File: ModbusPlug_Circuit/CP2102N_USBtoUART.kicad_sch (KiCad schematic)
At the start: 10 parts, among them U2 CP2102N-Axx-xQFN20

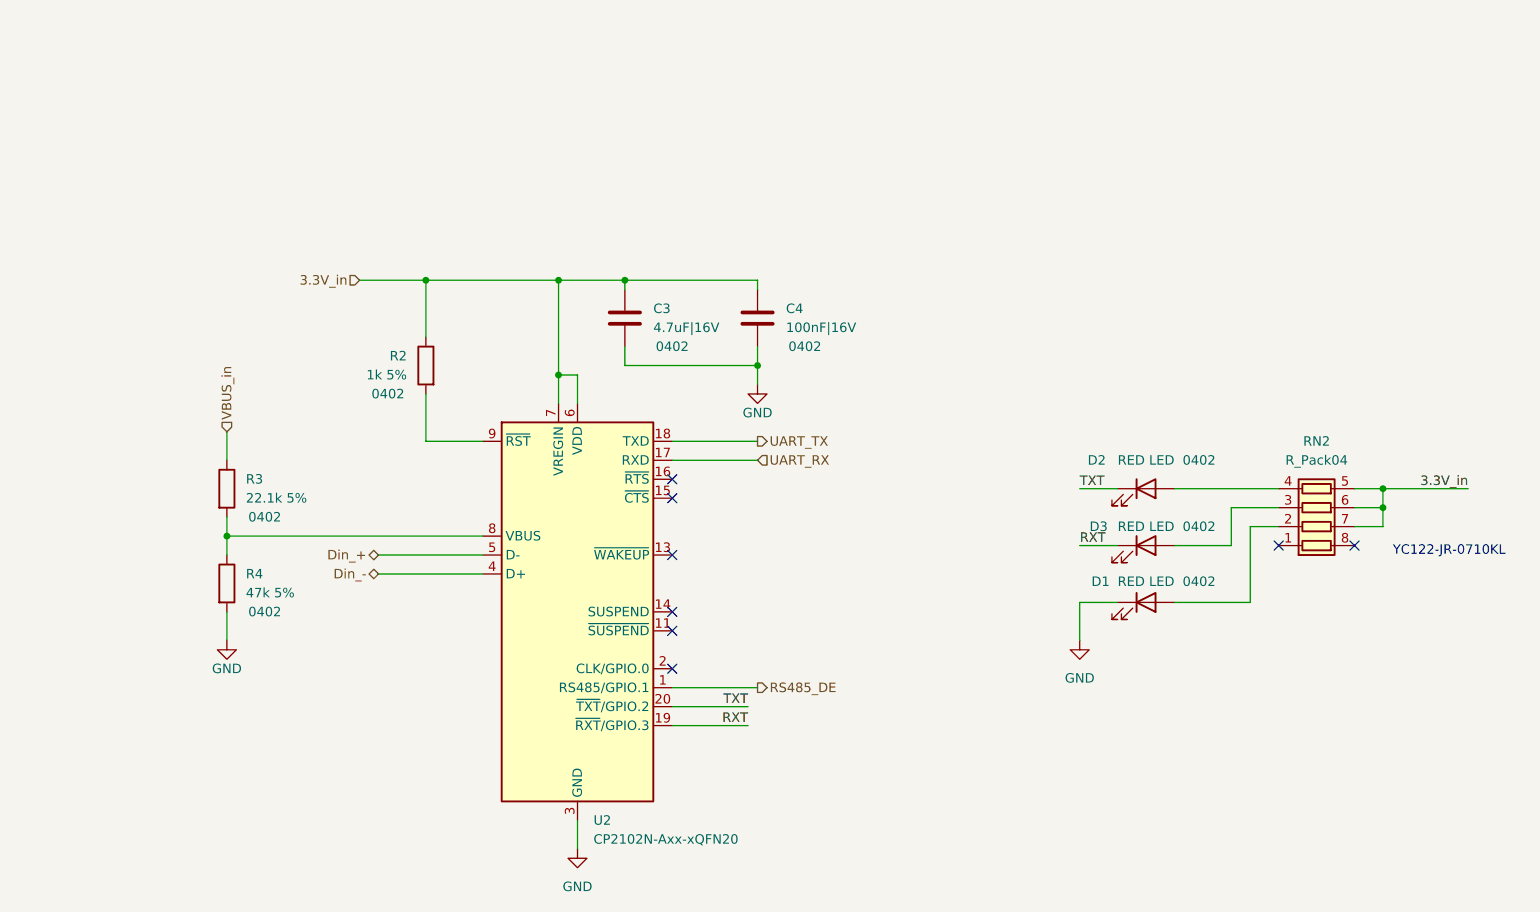
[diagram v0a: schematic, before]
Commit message: pushing V0.1.4
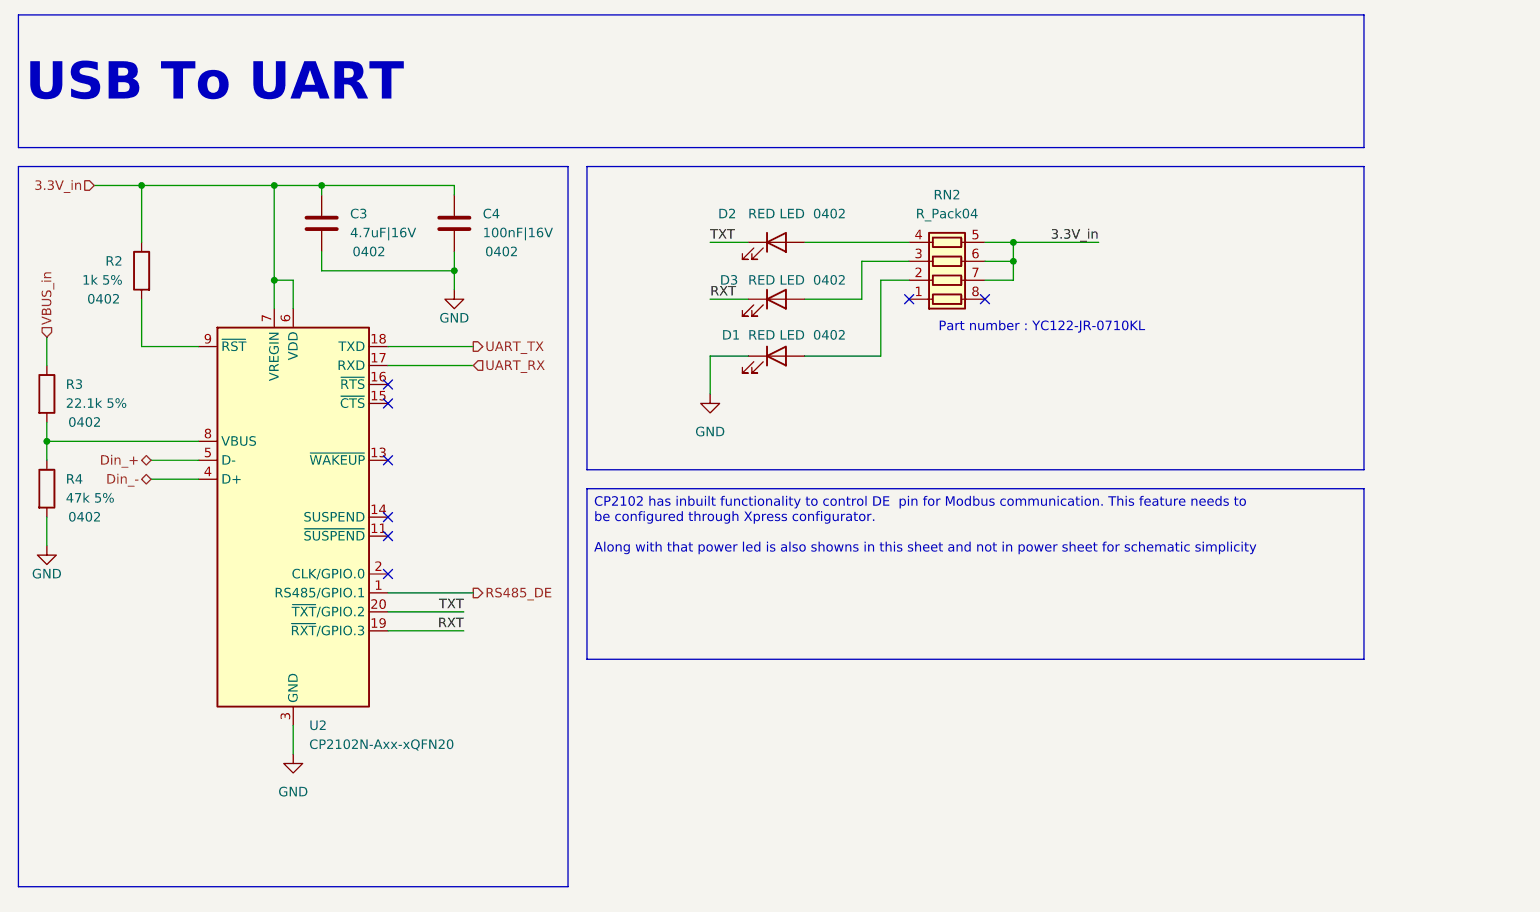
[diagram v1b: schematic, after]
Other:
- note added: "Part number : YC122-JR-0710KL"
- note removed: "YC122-JR-0710KL"
- title: (none) -> ModbusPlug
- moved on the sheet: C3, C4, D1, D2, D3, R2, R3, R4, RN2, U2
